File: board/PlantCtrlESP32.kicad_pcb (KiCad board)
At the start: 2 copper layers, 99.1 x 99.1 mm, 143 parts, among them IC1 DW01, J1 Conn_01x03_Female, J2 Conn_01x04, J3 Conn_01x04, J4 Conn_01x02_Female, J5 Conn_01x04, J6 Conn_01x03, J7 Conn_01x02, J8 Conn_01x02, Q1 N-channel 30V 5A, Q10 N-channel 30V 5A, Q11 N-channel 30V 5A, Q12 N-channel 30V 5A, Q2 N-channel 30V 5A, Q3 N-channel 30V 5A, Q4 N-channel 30V 5A, Q5 N-channel 30V 5A, Q6 N-channel 30V 5A, Q7 N-channel 30V 5A, Q8 N-channel 30V 5A, Q9 N-channel 30V 5A, U1 DS18B20, U2 ESP32-DEVKITC-32D, U3 LP38690DT-3.3, U4 SX1308

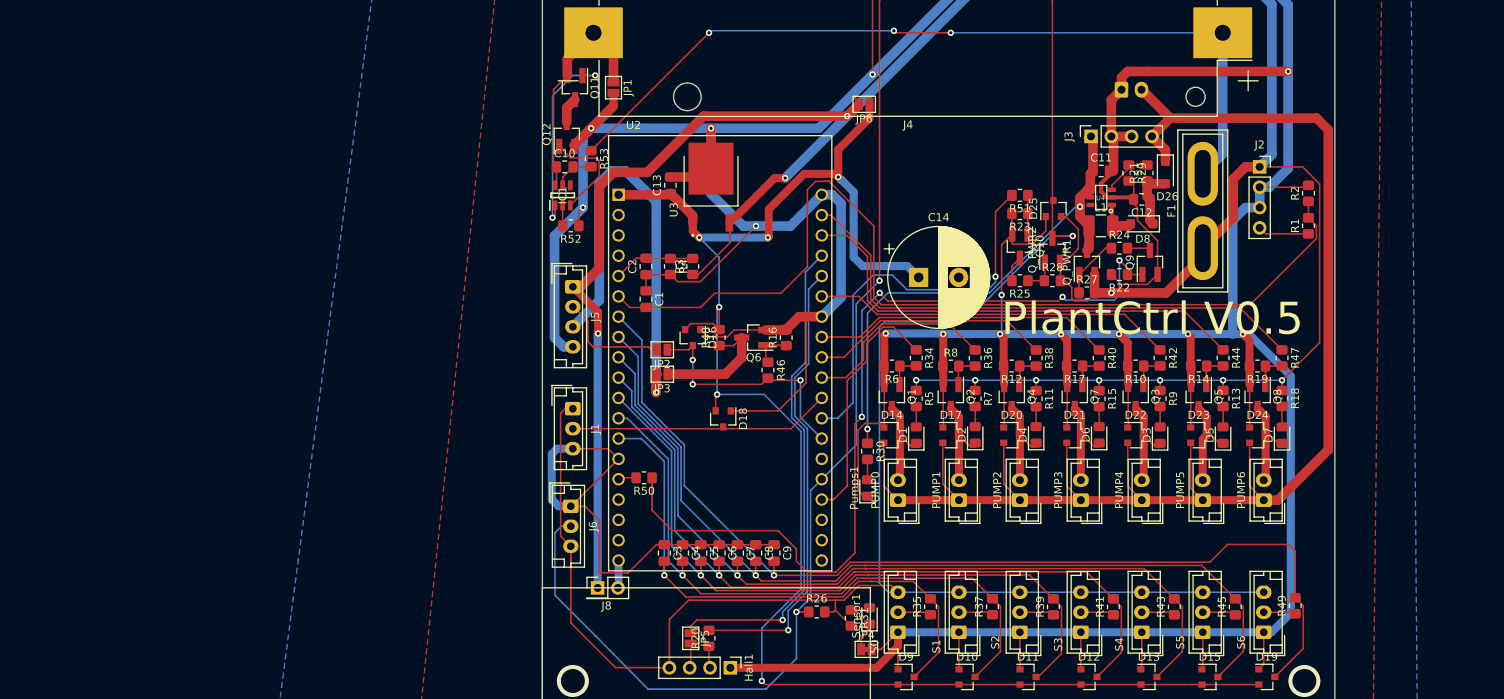
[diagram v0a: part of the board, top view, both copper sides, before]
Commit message: Fuse holder replaced
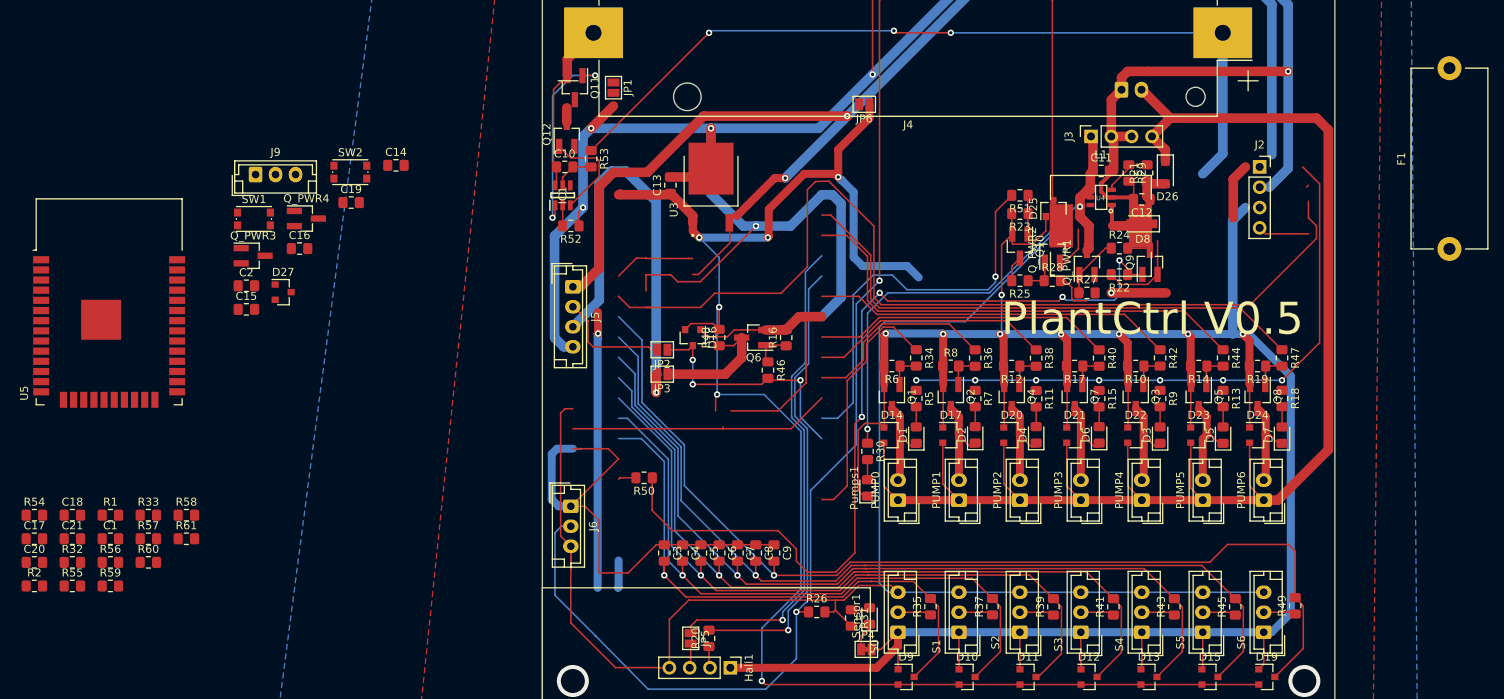
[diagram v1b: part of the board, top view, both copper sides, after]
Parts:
- removed D18: BAS40-04, Package_TO_SOT_SMD:SOT-23
- removed J1: Conn_01x03_Female, Connector_JST:JST_EH_B3B-EH-A_1x03_P2.50mm_Vertical
- removed J8: Conn_01x02, Connector_PinHeader_2.54mm:PinHeader_2x01_P2.54mm_Vertical
- removed R3: 33k, Resistor_SMD:R_0805_2012Metric_Pad1.20x1.40mm_HandSolder
- removed R4: 47k, Resistor_SMD:R_0805_2012Metric_Pad1.20x1.40mm_HandSolder
- removed U2: ESP32-DEVKITC-32D, ESP32:MODULE_ESP32-DEVKITC-32D
- added C15: 22uf, Capacitor_SMD:C_0805_2012Metric_Pad1.15x1.40mm_HandSolder, F.Cu at (133.2, 89.2)
- added C16: 22uf, Capacitor_SMD:C_0805_2012Metric_Pad1.15x1.40mm_HandSolder, F.Cu at (139.8, 81.6)
- added C17: 100n, Capacitor_SMD:C_0805_2012Metric_Pad1.15x1.40mm_HandSolder, F.Cu at (106.7, 117.9)
- added C18: 100n, Capacitor_SMD:C_0805_2012Metric_Pad1.15x1.40mm_HandSolder, F.Cu at (111.4, 114.9)
- added C19: 22uf, Capacitor_SMD:C_0805_2012Metric_Pad1.15x1.40mm_HandSolder, F.Cu at (146.3, 75.8)
- added C20: 1u, Capacitor_SMD:C_0805_2012Metric_Pad1.15x1.40mm_HandSolder, F.Cu at (106.7, 120.8)
- added C21: 1u, Capacitor_SMD:C_0805_2012Metric_Pad1.15x1.40mm_HandSolder, F.Cu at (111.4, 117.9)
- added D27: BAS40-04, Package_TO_SOT_SMD:SOT-23, F.Cu at (137.8, 87.0)
- added J9: Conn_01x03_Female, Connector_JST:JST_EH_B3B-EH-A_1x03_P2.50mm_Vertical, F.Cu at (134.3, 72.3)
- added Q_PWR3: P-channel 50v 4A, Package_TO_SOT_SMD:SOT-23_Handsoldering, F.Cu at (134.0, 82.5)
- added Q_PWR4: P-channel 50v 4A, Package_TO_SOT_SMD:SOT-23_Handsoldering, F.Cu at (140.7, 77.8)
- added R32: 10k, Resistor_SMD:R_0805_2012Metric_Pad1.15x1.40mm_HandSolder, F.Cu at (111.4, 120.8)
- added R33: 10k, Resistor_SMD:R_0805_2012Metric_Pad1.15x1.40mm_HandSolder, F.Cu at (120.9, 114.9)
- added R54: 33k, Resistor_SMD:R_0805_2012Metric_Pad1.15x1.40mm_HandSolder, F.Cu at (106.7, 114.9)
- added R55: 100k, Resistor_SMD:R_0805_2012Metric_Pad1.15x1.40mm_HandSolder, F.Cu at (111.4, 123.8)
- added R56: 47k, Resistor_SMD:R_0805_2012Metric_Pad1.15x1.40mm_HandSolder, F.Cu at (116.2, 120.8)
- added R57: 33k, Resistor_SMD:R_0805_2012Metric_Pad1.15x1.40mm_HandSolder, F.Cu at (120.9, 117.9)
- added R58: 10k, Resistor_SMD:R_0805_2012Metric_Pad1.15x1.40mm_HandSolder, F.Cu at (125.7, 114.9)
- added R59: 10k, Resistor_SMD:R_0805_2012Metric_Pad1.15x1.40mm_HandSolder, F.Cu at (116.2, 123.8)
- added R60: 10k, Resistor_SMD:R_0805_2012Metric_Pad1.15x1.40mm_HandSolder, F.Cu at (120.9, 120.8)
- added R61: 10k, Resistor_SMD:R_0805_2012Metric_Pad1.15x1.40mm_HandSolder, F.Cu at (125.7, 117.9)
- added SW1: SW_Push, Button_Switch_SMD:SW_Push_1P1T_NO_CK_KMR2, F.Cu at (134.1, 77.9)
- added SW2: SW_Push, Button_Switch_SMD:SW_Push_1P1T_NO_CK_KMR2, F.Cu at (146.2, 72.0)
- added U5: ESP32-WROOM-32D, RF_Module:ESP32-WROOM-32, F.Cu at (116.0, 91.2)
- C1: value 1u -> 100n; footprint Capacitor_SMD:C_0805_2012Metric_Pad1.18x1.45mm_HandSolder -> Capacitor_SMD:C_0805_2012Metric_Pad1.15x1.40mm_HandSolder
- C10, C3, C4, C5, C6, C7, C8, C9: footprint Capacitor_SMD:C_0805_2012Metric_Pad1.18x1.45mm_HandSolder -> Capacitor_SMD:C_0805_2012Metric_Pad1.15x1.40mm_HandSolder
- C14: value 100u -> 22uf; footprint Capacitor_THT:CP_Radial_D12.5mm_P5.00mm -> Capacitor_SMD:C_0805_2012Metric_Pad1.15x1.40mm_HandSolder
- C2: value 1u -> 22uf; footprint Capacitor_SMD:C_0805_2012Metric_Pad1.18x1.45mm_HandSolder -> Capacitor_SMD:C_0805_2012Metric_Pad1.15x1.40mm_HandSolder
- F1: footprint Fuse:Fuse_Blade_ATO_directSolder -> Fuse:Fuseholder_Cylinder-5x20mm_Stelvio-Kontek_PTF78_Horizontal_Open
- JP5: value SolderJumper_2_Open -> Open
- L1: footprint Inductor_SMD:L_1210_3225Metric_Pad1.42x2.65mm_HandSolder -> Inductor_SMD:L_12x12mm_H4.5mm
- R1: value 100k -> 10k; footprint Resistor_SMD:R_0805_2012Metric_Pad1.20x1.40mm_HandSolder -> Resistor_SMD:R_0805_2012Metric_Pad1.15x1.40mm_HandSolder
- R10, R11, R12, R13, R14, R15, R16, R17, R18, R19, R20, R21, R22, R23, R24, R25, R26, R27, R28, R29, R30, R31, R34, R35, R36, R37, R38, R39, R40, R41, R42, R43, R44, R45, R46, R47, R48, R49, R5, R50, R51, R52, R53, R6, R7, R9: footprint Resistor_SMD:R_0805_2012Metric_Pad1.20x1.40mm_HandSolder -> Resistor_SMD:R_0805_2012Metric_Pad1.15x1.40mm_HandSolder
- R2: value 33k -> 10k; footprint Resistor_SMD:R_0805_2012Metric_Pad1.20x1.40mm_HandSolder -> Resistor_SMD:R_0805_2012Metric_Pad1.15x1.40mm_HandSolder
- U4: footprint SOT-23-6 -> misc_footprints:SOT-23-6
- moved R2 166.6 mm to (106.7, 123.8), turned to 0 degrees
- moved R1 154.1 mm to (116.2, 114.9), turned to 0 degrees
- moved C1 73.3 mm to (116.2, 117.9), turned to 0 degrees
- moved C14 66.8 mm to (151.9, 71.2)
- moved C2 50.0 mm to (133.2, 86.2), turned to 0 degrees
- moved F1 30.8 mm to (283.6, 81.6)
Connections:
- C14 pad 1: 3_3V -> PUMP_PWR
- C2 pad 2: Net-(C2-Pad2) -> IO0
- D25 pad 2: LIPO+ -> VCC
- F1 pad 1: LIPO+ -> Net-(F1-Pad1)
- J2 pad 1: LIPO+ -> Net-(F1-Pad1)
- J2 pad 2: GND -> Net-(J2-Pad2)
- J2 pad 3: GND -> Net-(J2-Pad2)
- J2 pad 4: SOLAR_IN -> Net-(J2-Pad4)
- J5 pad 1: LIPO+ -> VCC
- JP1 pad 1: GND_BATT -> Net-(J2-Pad2)
- JP1 pad 2: GND -> GND_BATT
- JP6 pad 2: LIPO+ -> VCC
- Q11 pad 3: Net-(Q11-Pad3) -> enable_all
- Q12 pad 2: GND -> Net-(J2-Pad2)
- Q12 pad 3: Net-(Q11-Pad3) -> GND_BATT
- Q_PWR1 pad 2: LIPO+ -> VCC
- Q_PWR2 pad 2: LIPO+ -> VCC
- R1 pad 1: SOLAR_IN -> IO0
- R11 pad 1: LIPO+ -> VCC
- R13 pad 1: LIPO+ -> VCC
- R15 pad 1: LIPO+ -> VCC
- R18 pad 1: LIPO+ -> VCC
- R2 pad 1: Net-(C1-Pad2) -> IO0
- R2 pad 2: GND -> 3_3V
- R27 pad 2: LIPO+ -> VCC
- R28 pad 2: LIPO+ -> VCC
- R5 pad 1: LIPO+ -> VCC
- R7 pad 1: LIPO+ -> VCC
- R9 pad 1: LIPO+ -> VCC
- U3 pad 3: LIPO+ -> VCC
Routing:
- net LIPO+: track 341.4 -> 288.0 mm
- net GND: track 763.2 -> 740.4 mm
- net PWR_SENSORS: track 250.4 -> 242.9 mm, vias 1 -> 0
- net SOLAR_IN: track 6.41 -> 0.00 mm
- net Net-(J2-Pad4): track 0.00 -> 6.41 mm
- net Net-(Q11-Pad3): track 3.26 -> 0.00 mm
- net Net-(C12-Pad1): track 8.09 -> 4.88 mm
- net GND_BATT: track 28.5 -> 26.7 mm

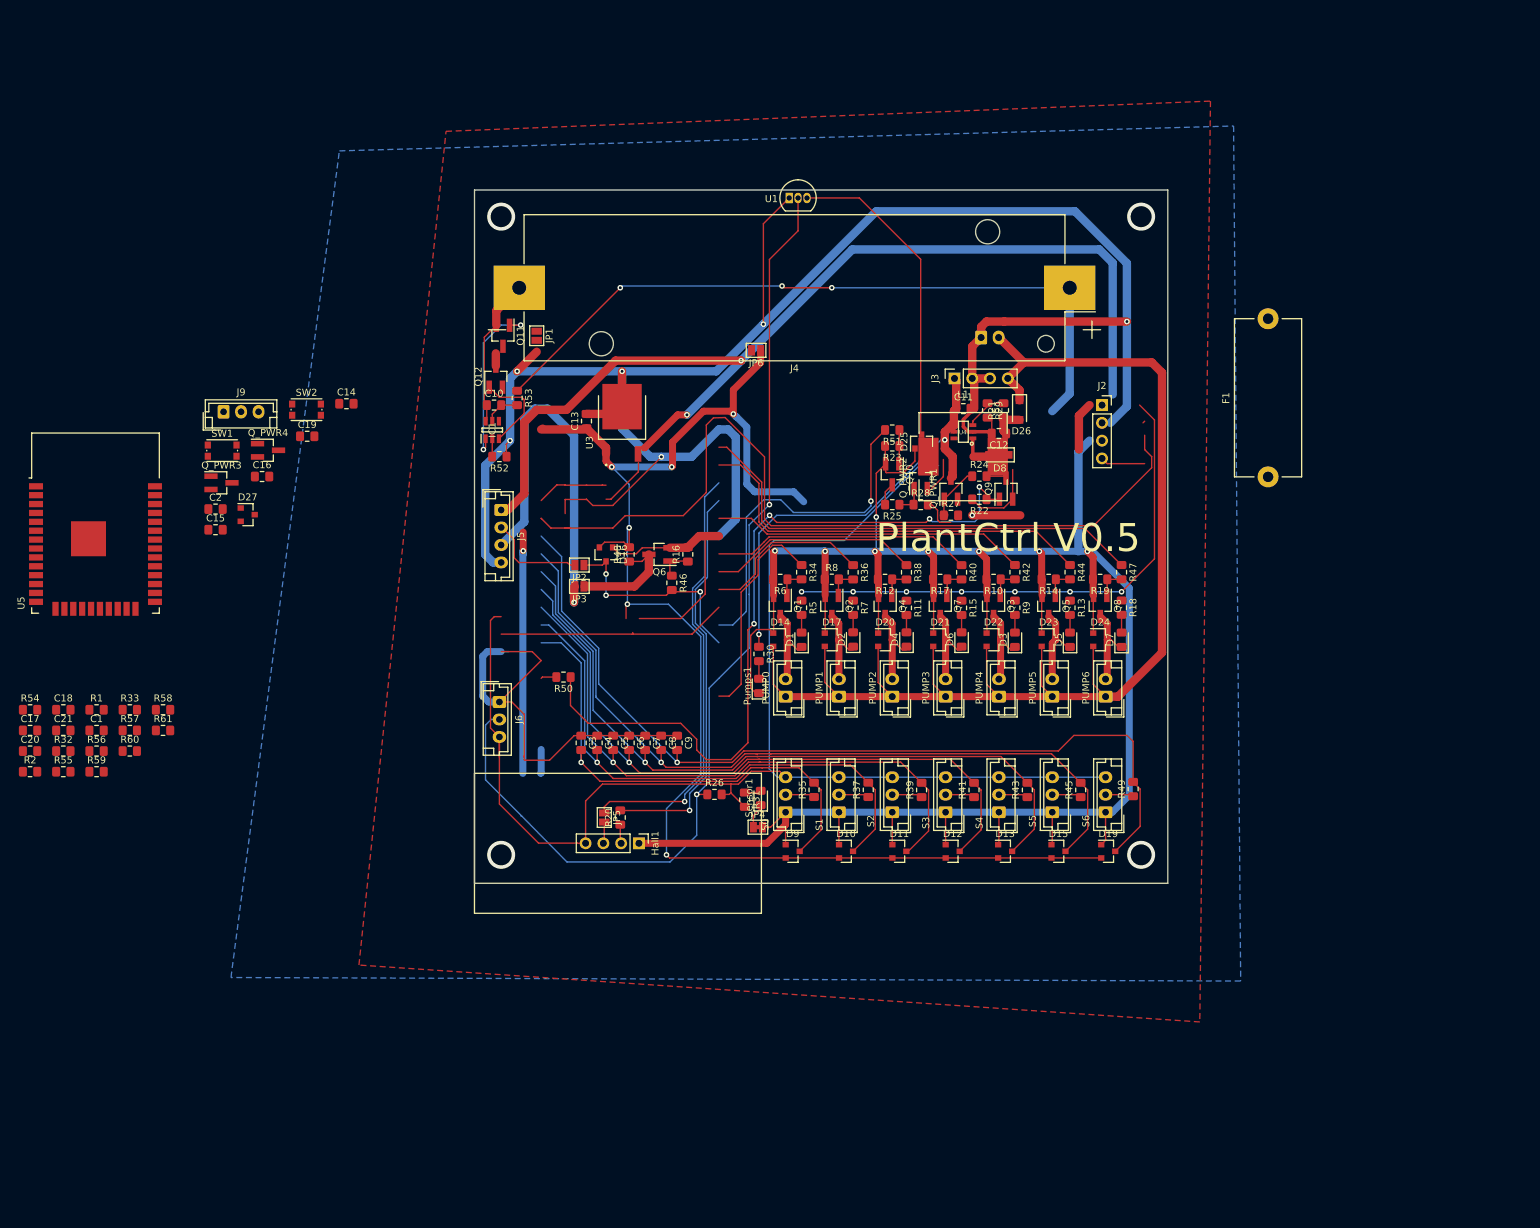
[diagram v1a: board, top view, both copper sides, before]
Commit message: updated pcb
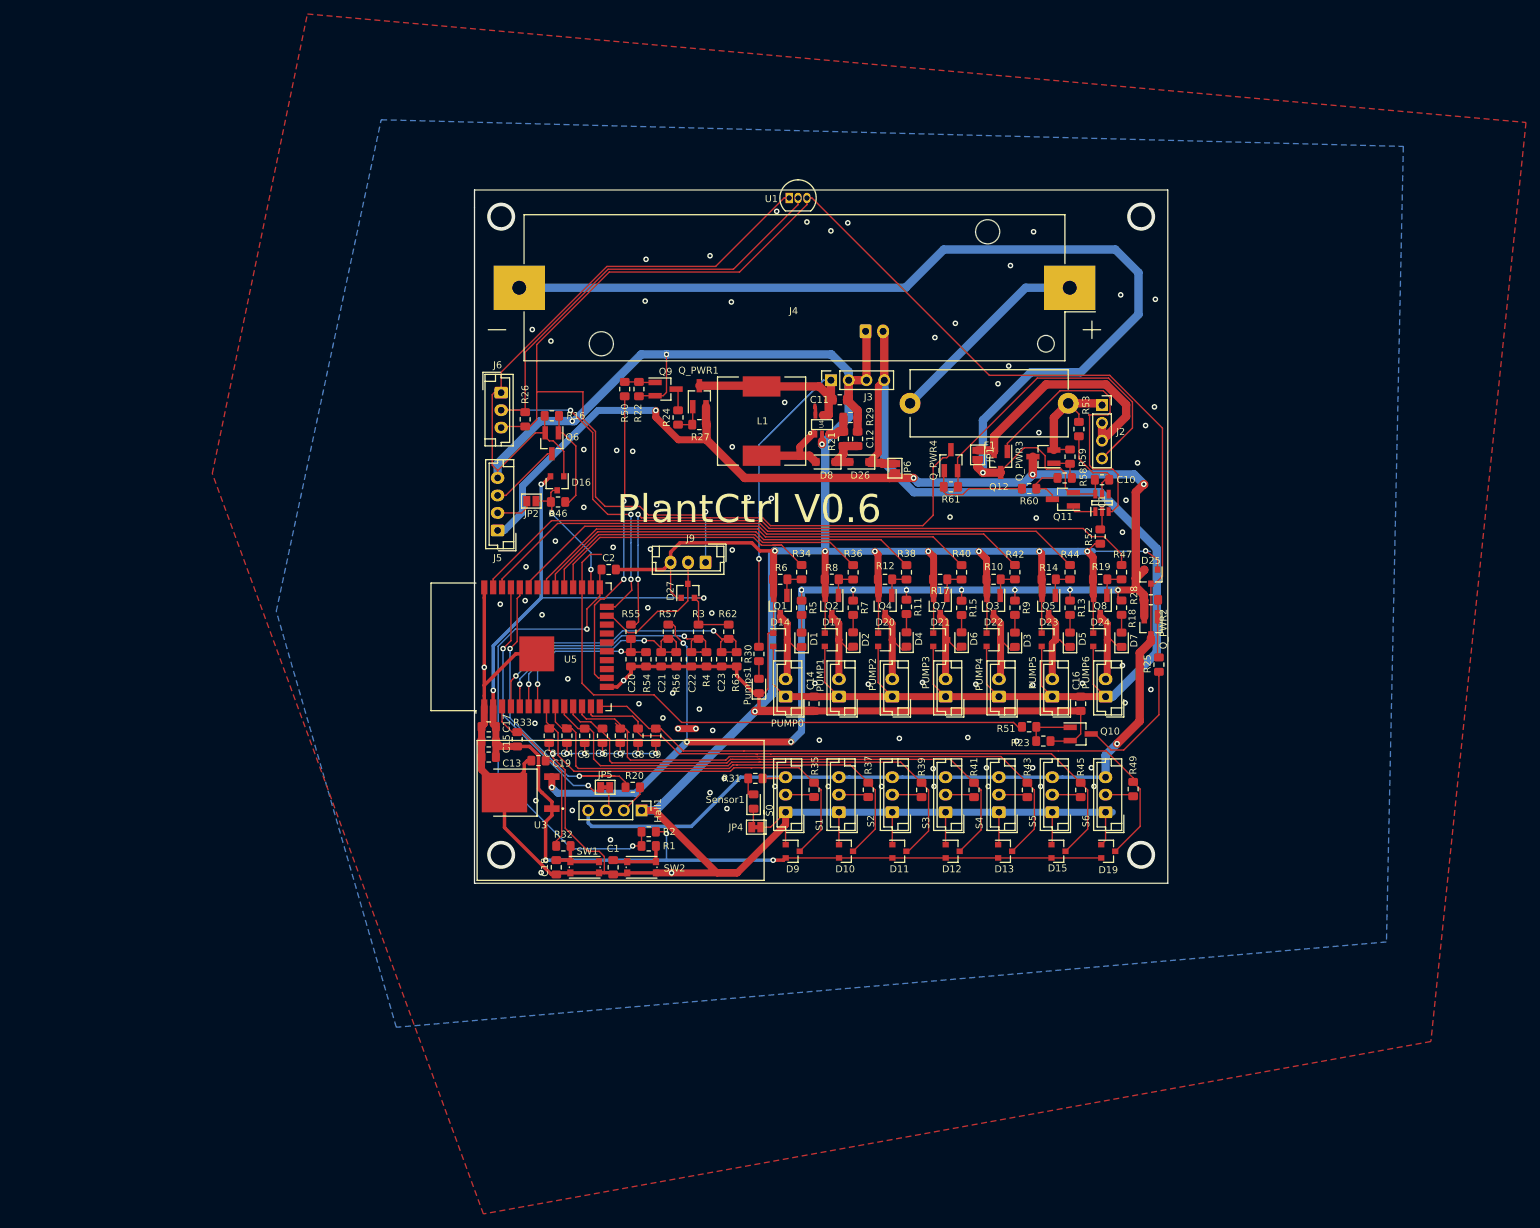
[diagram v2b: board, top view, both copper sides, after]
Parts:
- removed JP3: SolderJumper_2_Open, Jumper:SolderJumper-2_P1.3mm_Open_Pad1.0x1.5mm
- removed R48: 10k, Resistor_SMD:R_0805_2012Metric_Pad1.15x1.40mm_HandSolder
- added C22: 100n, Capacitor_SMD:C_0805_2012Metric_Pad1.15x1.40mm_HandSolder, F.Cu at (201.2, 107.7)
- added C23: 100n, Capacitor_SMD:C_0805_2012Metric_Pad1.15x1.40mm_HandSolder, F.Cu at (205.5, 107.7)
- added R3: 10k, Resistor_SMD:R_0805_2012Metric_Pad1.15x1.40mm_HandSolder, F.Cu at (202.2, 103.8)
- added R4: 33k, Resistor_SMD:R_0805_2012Metric_Pad1.15x1.40mm_HandSolder, F.Cu at (203.3, 107.7)
- added R62: 10k, Resistor_SMD:R_0805_2012Metric_Pad1.15x1.40mm_HandSolder, F.Cu at (206.5, 103.8)
- added R63: 10k, Resistor_SMD:R_0805_2012Metric_Pad1.15x1.40mm_HandSolder, F.Cu at (207.6, 107.7)
- added REF**: CCC_Mannheim_Logo2_full, ESP32:CCC_Mannheim_Logo2_full, B.Cu at (262.9, 82.0)
- added REF**: WEEE-Logo_5.6x8mm_SilkScreen, Symbol:WEEE-Logo_5.6x8mm_SilkScreen, B.Cu at (209.6, 134.9)
- added REF**: FCC-Logo_9.6x8mm_SilkScreen, Symbol:FCC-Logo_9.6x8mm_SilkScreen, B.Cu at (201.0, 133.0)
- added REF**: CE-Logo_16.8x12mm_SilkScreen, Symbol:CE-Logo_16.8x12mm_SilkScreen, B.Cu at (185.9, 131.4)
- JP4: value SolderJumper_2_Open -> NC
- JP5: value Open -> NC; footprint Jumper:SolderJumper-2_P1.3mm_Open_Pad1.0x1.5mm -> Jumper:SolderJumper-2_P1.3mm_Bridged_Pad1.0x1.5mm
- moved R59 146.2 mm to (255.3, 78.7), turned to 90 degrees
- moved R60 133.9 mm to (249.4, 83.3)
- moved R58 133.0 mm to (254.5, 81.8), turned to 180 degrees
- moved C16 121.4 mm to (256.8, 114.0), turned to 270 degrees
- moved R61 117.8 mm to (238.3, 83.1)
- moved Q_PWR3 117.5 mm to (251.5, 78.7), turned to 180 degrees
- moved Q_PWR4 97.6 mm to (238.3, 79.2), turned to 90 degrees
- moved R2 88.8 mm to (195.1, 132.3)
- moved R54 88.3 mm to (194.7, 107.7), turned to 270 degrees
- moved IC1 87.7 mm to (259.8, 85.3)
- moved C10 87.5 mm to (259.8, 82.0)
- moved C20 86.8 mm to (192.5, 107.7), turned to 90 degrees
- moved R52 86.6 mm to (259.6, 90.2), turned to 90 degrees
- moved C21 86.0 mm to (196.8, 107.7), turned to 90 degrees
- moved R56 83.9 mm to (199.0, 107.7), turned to 270 degrees
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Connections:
- JP6 pad 1: 3_3V -> PUMP_PWR
- Q6 pad 3: Net-(JP3-Pad1) -> Net-(J5-Pad3)
- R53 pad 1: VCC_BATT -> Net-(F1-Pad1)
- U5 pad 10: PLANT4_MOIST -> PLANT2_MOIST
- U5 pad 12: PLANT2_MOIST -> PLANT4_MOIST
- U5 pad 13: PLANT1_MOIST -> PLANT5_MOIST
- U5 pad 14: PLANT0_MOIST -> PLANT6_MOIST
- U5 pad 23: PLANT_CTRL_PUMP_0 -> Net-(D27-Pad3)
- U5 pad 28: Net-(D27-Pad3) -> PLANT_CTRL_PUMP_0
- U5 pad 4: (no net) -> Net-(C23-Pad2)
- U5 pad 5: (no net) -> Net-(C22-Pad2)
- U5 pad 8: PLANT6_MOIST -> PLANT0_MOIST
- U5 pad 9: PLANT5_MOIST -> PLANT1_MOIST
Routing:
- net LIPO+: track 288.0 -> 0.00 mm, vias 11 -> 0
- net VCC: track 0.00 -> 279.0 mm, vias 0 -> 15
- net GND_BATT: track 26.7 -> 164.4 mm, vias 0 -> 1
- net PWR_SENSORS: track 242.9 -> 359.4 mm, vias 0 -> 2
- net Net-(C1-Pad2): track 120.9 -> 8.46 mm
- net Net-(Q9-Pad1): track 107.8 -> 4.37 mm, vias 4 -> 0
- net VCC_BATT: track 103.9 -> 29.7 mm, vias 3 -> 0
- net SOLAR_IN: track 0.00 -> 70.8 mm, vias 0 -> 2
- net IO0: track 0.00 -> 68.5 mm, vias 0 -> 2
- net Net-(C23-Pad2): track 0.00 -> 45.8 mm, vias 0 -> 2
- net Net-(J5-Pad3): track 54.9 -> 10.2 mm, vias 1 -> 0
- net Net-(J2-Pad4): track 6.41 -> 48.4 mm
- net PUMP_ENABLE: track 2.27 -> 43.8 mm, vias 0 -> 2
- net Net-(C22-Pad2): track 0.00 -> 39.7 mm, vias 0 -> 2
- net GND: track 740.4 -> 779.0 mm, vias 14 -> 105
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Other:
- board text added: "PlantCtrl V0.6"
- board text removed: "PlantCtrl V0.5"
